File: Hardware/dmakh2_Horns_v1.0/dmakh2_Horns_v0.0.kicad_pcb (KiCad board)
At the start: 2 copper layers, 51 x 30 mm, 17 parts, among them J1 Conn_01x03, J2 Conn_01x02, J3 HORN2, J4 HORN1, Q1 IRLZ44N

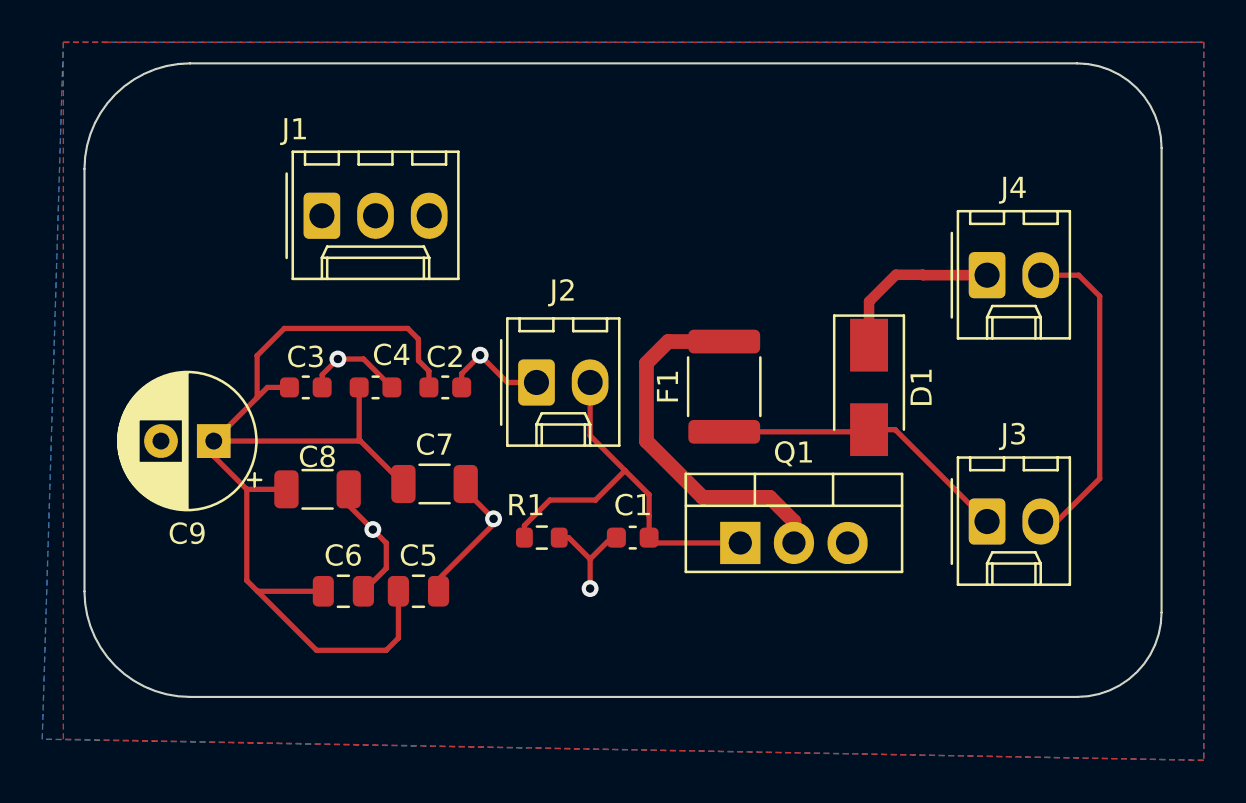
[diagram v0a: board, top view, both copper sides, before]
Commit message: pushing 2 mini projects and hardware challenge project
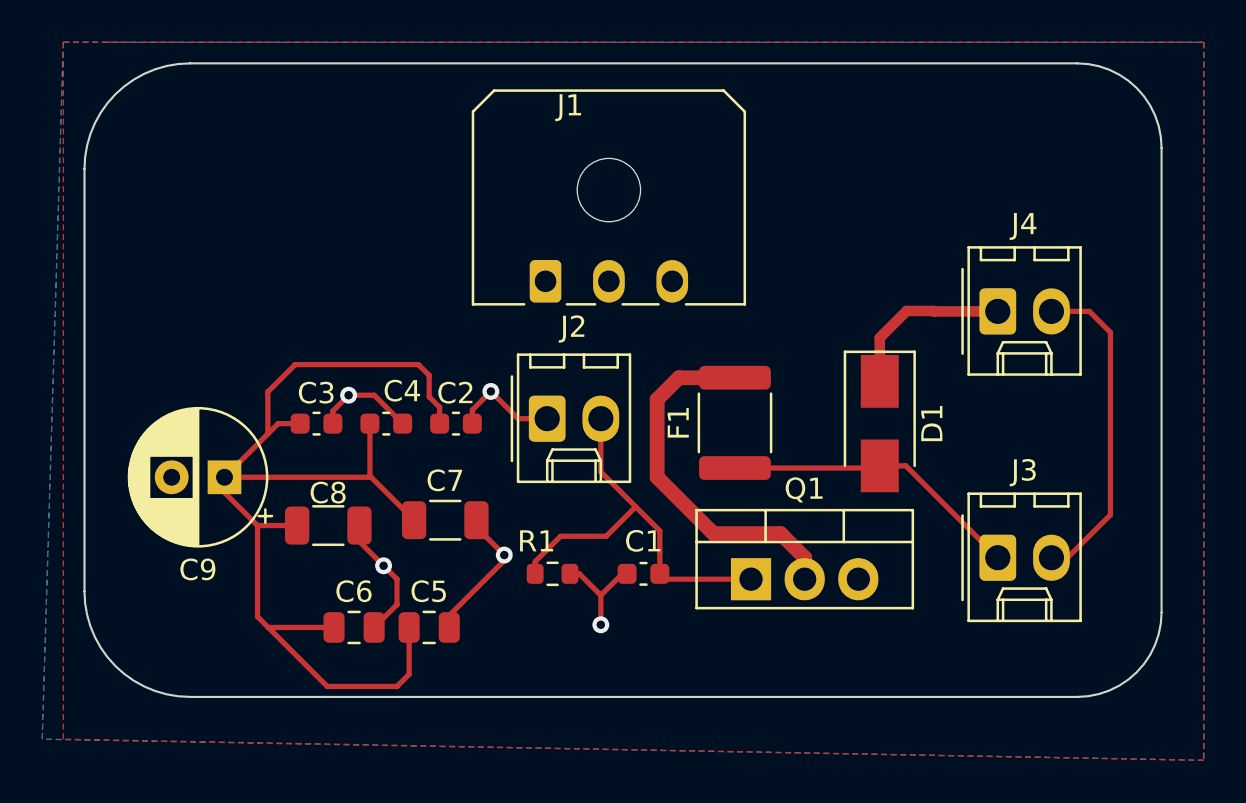
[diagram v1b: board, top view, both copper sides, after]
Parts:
- J1: footprint Connector_Molex:Molex_KK-254_AE-6410-03A_1x03_P2.54mm_Vertical -> Connector_Molex:Molex_Micro-Fit_3.0_43650-0300_1x03_P3.00mm_Horizontal
- moved J1 11.0 mm to (168.8, 80.3)
- moved C2 1.79 mm to (164.6, 87.1)
- moved C3 1.79 mm to (158.0, 87.1)
- moved C5 1.79 mm to (163.3, 96.7)
- moved C7 1.79 mm to (164.1, 91.6)
- moved F1 1.79 mm to (177.8, 87.0)
- moved J2 1.79 mm to (168.9, 86.8)
- moved J3 1.79 mm to (190.2, 93.4)
- moved J4 1.79 mm to (190.2, 81.7)
- moved Q1 1.79 mm to (178.6, 94.4)
- moved C1 1.79 mm to (173.5, 94.2)
- moved C4 1.79 mm to (161.3, 87.1)
- moved C6 1.79 mm to (159.8, 96.7)
- moved C8 1.79 mm to (158.5, 91.9)
- moved C9 1.79 mm to (153.6, 89.6)
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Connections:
- J1 pad 3: GND -> (no net)
